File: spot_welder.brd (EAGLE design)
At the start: 77 x 53.8 mm, 38 parts, among them IC1 ATMEGA328PU, IC2 7805L, IC3 MOC3052M, T1 BT151-800R, T2 BT151-800R, Y1 16MHZ

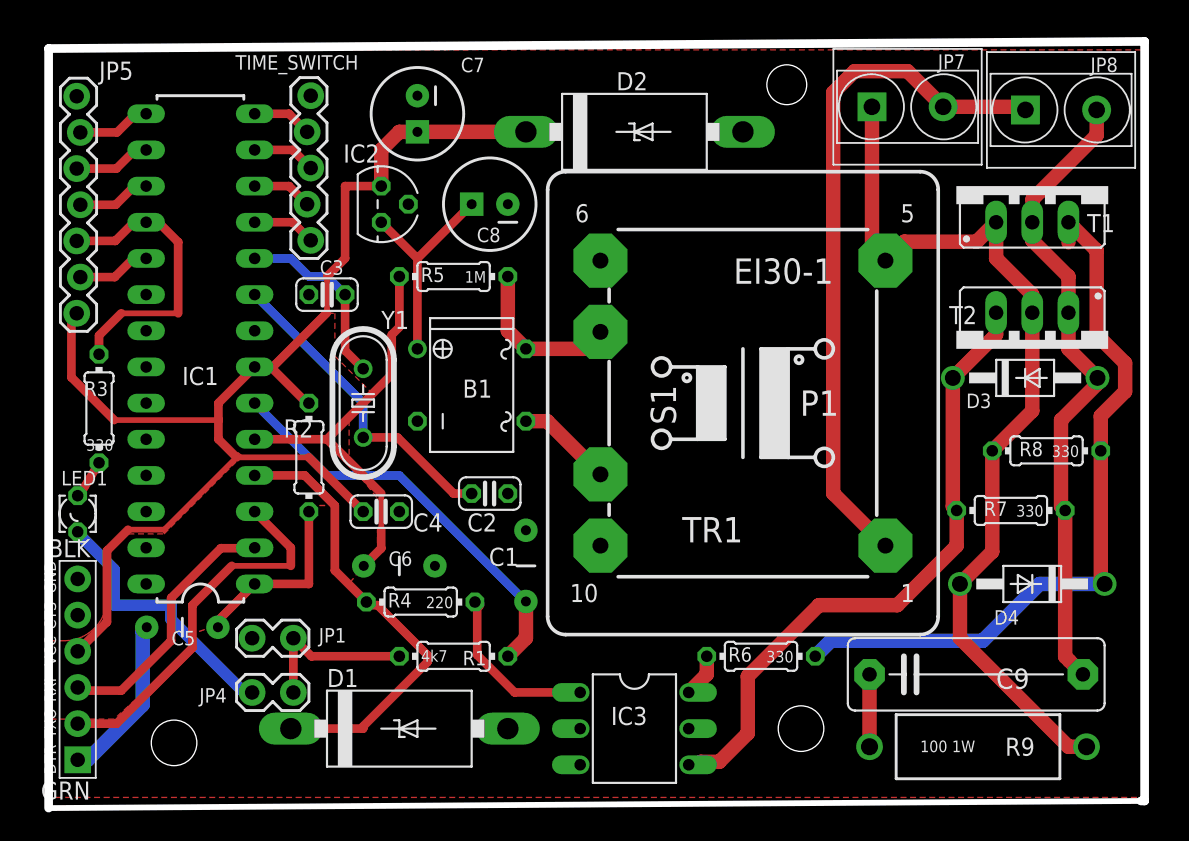
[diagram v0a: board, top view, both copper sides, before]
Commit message: rerouted
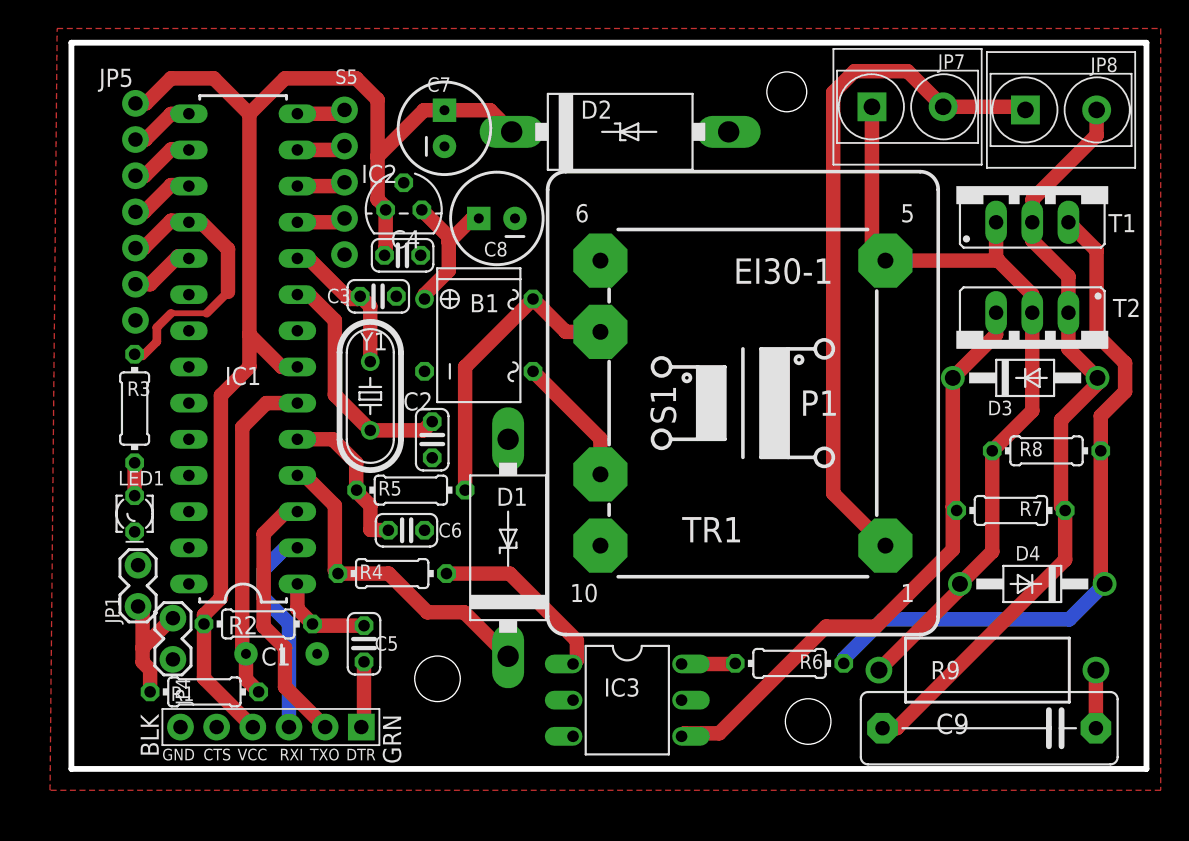
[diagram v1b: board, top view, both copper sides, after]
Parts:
- removed TIME_SWITCH: Time switch, SparkFun-Connectors:1X05_LOCK
- added S5: Time switch, SparkFun-Connectors:1X05_NO_SILK
- C5, C6: device SparkFun-Passives:CAP-PTH-5MM -> rcl:C025-024X044
- JP5: device SparkFun-Connectors:1X07_LOCK -> SparkFun-Connectors:1X07_NO_SILK
- moved C1 18.2 mm to (41.3, 42.1), turned to 0 degrees
- moved C4 18.1 mm to (49.8, 70.1)
- moved R1 17.7 mm to (35.8, 39.4)
- moved R5 15.3 mm to (50.3, 53.6)
- moved D1 14.8 mm to (57.2, 49.5), turned to 90 degrees
- moved JP2 14.2 mm to (40.5, 36.9), turned to 180 degrees
- moved C5 12.8 mm to (47.0, 42.8), turned to 90 degrees
- moved R2 12.2 mm to (39.6, 44.2), turned to 0 degrees
- moved JP1 11.0 mm to (31.2, 45.6), turned to 90 degrees
- moved JP4 6.26 mm to (33.6, 41.9), turned to 90 degrees
- moved C2 5.53 mm to (51.8, 57.1), turned to 90 degrees
- moved R9 5.42 mm to (90.8, 40.9), turned to 180 degrees
- moved JP5 4.03 mm to (31.0, 65.5)
- moved LED1 4.00 mm to (30.9, 51.9)
- moved C9 3.89 mm to (91.0, 36.9), turned to 180 degrees
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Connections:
- net GND: now also JP5.1, S5.5; no longer JP5.7, TIME_SWITCH.1
- net N$18: now also S5.4; no longer TIME_SWITCH.5
- net N$23: now also S5.3; no longer TIME_SWITCH.4
- net N$24: now also S5.2; no longer TIME_SWITCH.3
- net N$25: now also S5.1; no longer TIME_SWITCH.2
- net VCC: now also JP5.7; no longer JP5.1
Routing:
- net GND: track 19.2 -> 0.00 mm
- net N$13: track 29.6 -> 11.2 mm
- net N$10: track 66.2 -> 56.2 mm
- net N$1: track 11.3 -> 21.1 mm
- net N$15: track 32.1 -> 22.7 mm
- net N$3: track 45.1 -> 54.3 mm
- net N$19: track 26.2 -> 18.4 mm
- net N$7: track 11.7 -> 4.66 mm
- net N$14: track 13.0 -> 6.92 mm
- net N$16: track 22.4 -> 16.7 mm
- net N$22: track 29.2 -> 23.6 mm
- net N$2: track 15.3 -> 10.5 mm
- net N$20: track 18.4 -> 14.8 mm
- net VCC: track 89.9 -> 93.1 mm
- net N$6: track 45.9 -> 42.8 mm
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- removed copper zone on layer 1, net VCC
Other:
- board size 77 x 53.8 mm -> 75.5 x 51 mm
